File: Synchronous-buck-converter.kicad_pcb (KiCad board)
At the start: 2 copper layers, 107.2 x 56.3 mm, 84 parts, among them IC1 2EDF7275FXUMA2, IC2 LM5169PQDDARQ1, J1 Conn_01x02_Socket, J2 output, J4 RP2040 connector, Q1 IPP50R280CE, Q2 IPP50R280CE, U1 MGJ2D151505SC, U2 MGJ2D151505SC, U4 3.3V reg

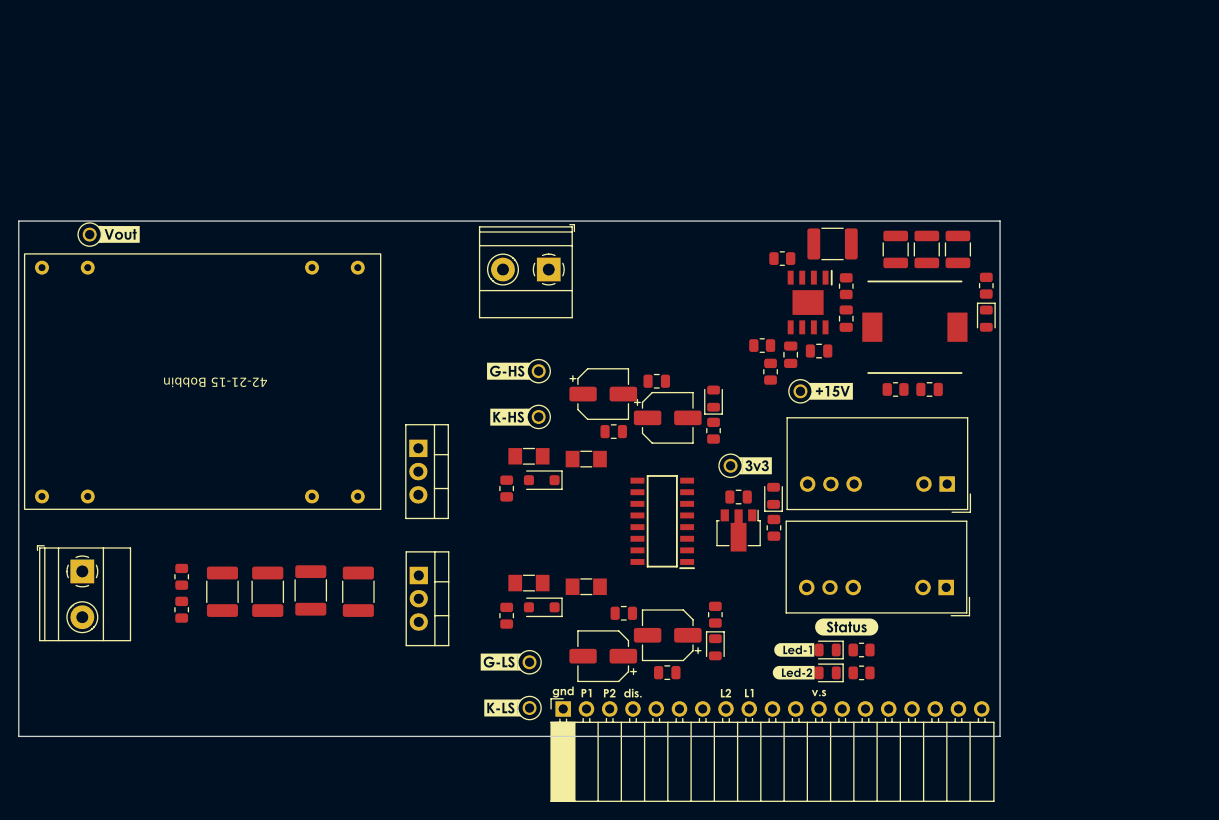
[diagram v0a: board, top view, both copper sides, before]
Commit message: V1
layout and tracing done
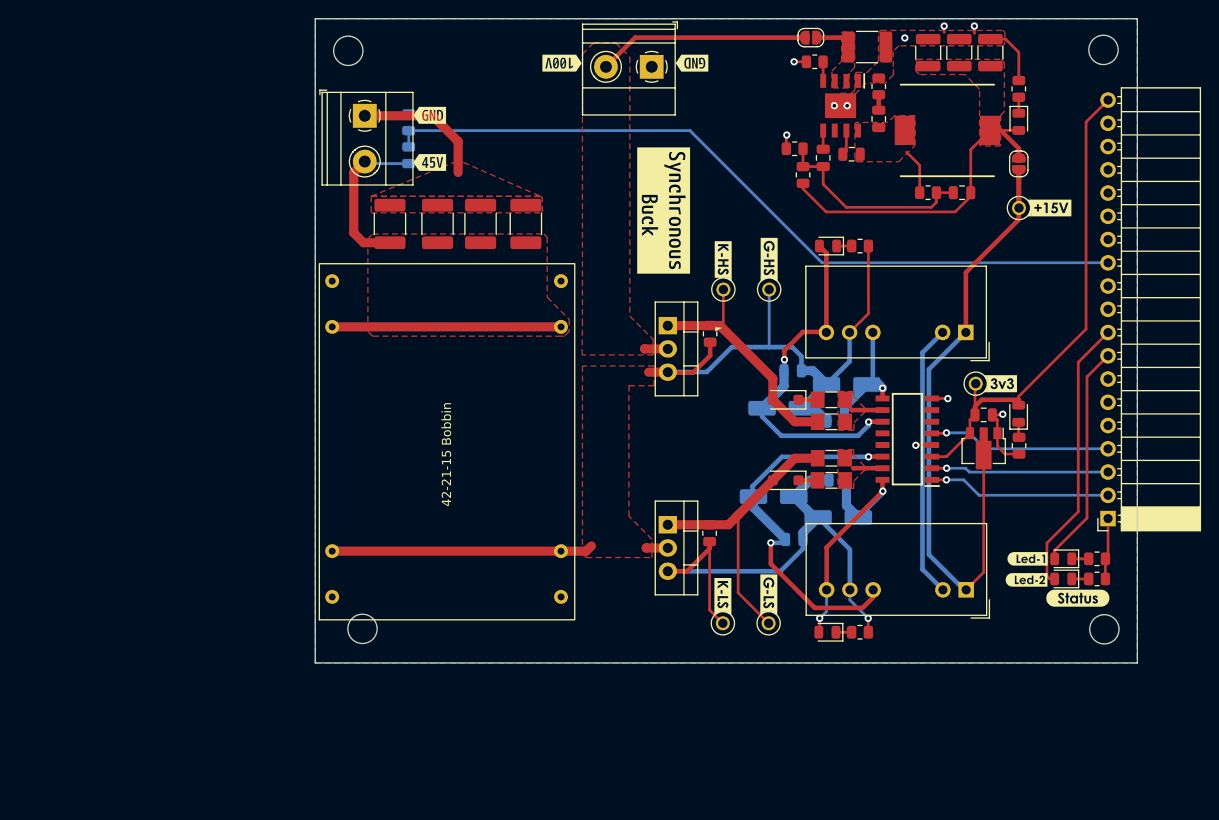
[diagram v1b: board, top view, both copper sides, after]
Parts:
- removed TP5: Vout, 5001 tp:KEYSTONE_5001
- removed kibuzzard-65CA698D: G***, kibuzzard-65CA698D
- removed kibuzzard-65CA6A14: G***, kibuzzard-65CA6A14
- removed kibuzzard-65CA6A3B: G***, kibuzzard-65CA6A3B
- removed kibuzzard-65CA6A4E: G***, kibuzzard-65CA6A4E
- removed kibuzzard-65CA6AA3: G***, kibuzzard-65CA6AA3
- removed kibuzzard-65CA6AAA: G***, kibuzzard-65CA6AAA
- removed kibuzzard-65CA6ABB: G***, kibuzzard-65CA6ABB
- removed kibuzzard-65CA6B07: G***, kibuzzard-65CA6B07
- added H1: MountingHole, MountingHole:MountingHole_3.2mm_M3, F.Cu at (120.0, 134.1)
- added H2: MountingHole, MountingHole:MountingHole_3.2mm_M3, F.Cu at (201.1, 134.1)
- added H3: MountingHole, MountingHole:MountingHole_3.2mm_M3, F.Cu at (118.5, 70.9)
- added H4: MountingHole, MountingHole:MountingHole_3.2mm_M3, F.Cu at (201.0, 70.8)
- added JP1: jumper, Jumper:SolderJumper-2_P1.3mm_Open_RoundedPad1.0x1.5mm, F.Cu at (169.0, 69.5)
- added JP2: jumper, Jumper:SolderJumper-2_P1.3mm_Open_RoundedPad1.0x1.5mm, F.Cu at (191.8, 83.2)
- added kibuzzard-65F43C21: G***, kibuzzard-65F43C21, F.Cu at (152.9, 88.3)
- added kibuzzard-65F43C4A: G***, kibuzzard-65F43C4A, F.Cu at (141.8, 72.2)
- added kibuzzard-65F43C74: G***, kibuzzard-65F43C74, F.Cu at (156.1, 72.2)
- added kibuzzard-65F43CE0: G***, kibuzzard-65F43CE0, F.Cu at (127.4, 83.1)
- added kibuzzard-65F43CF3: G***, kibuzzard-65F43CF3, F.Cu at (127.4, 78.0)
- added kibuzzard-65F44031: G***, kibuzzard-65F44031, F.Cu at (146.6, 88.3)
- added kibuzzard-65F4406D: G***, kibuzzard-65F4406D, F.Cu at (146.6, 116.5)
- C12, C13, C14, C15, C16, C17, C18, C19, R7, R8: moved to B.Cu
- moved J4 63.0 mm to (201.5, 122.0), turned to 180 degrees
- moved R8 58.7 mm to (125.1, 78.7), turned to 90 degrees
- moved J2 58.6 mm to (120.3, 78.0)
- moved R7 52.3 mm to (125.1, 82.3), turned to 90 degrees
- moved C4 52.1 mm to (137.9, 89.8), turned to 90 degrees
- moved C3 46.4 mm to (132.9, 89.8), turned to 90 degrees
- moved L1 45.2 mm to (143.2, 133.1), turned to 90 degrees
- moved C2 42.4 mm to (128.2, 89.8), turned to 90 degrees
- moved C1 40.3 mm to (123.0, 89.8), turned to 90 degrees
- moved R1 35.7 mm to (171.3, 115.4)
- moved R5 33.3 mm to (171.3, 111.4)
- moved kibuzzard-65CA6838 31.2 mm to (164.5, 93.5), turned to -90 degrees
- moved TP6 31.2 mm to (191.8, 88.1)
- moved kibuzzard-65CA6608 31.2 mm to (195.3, 88.1)
- moved kibuzzard-65CA6739 30.4 mm to (164.4, 130.1), turned to -90 degrees
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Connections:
- C1 pad 1: Net-(J2-Pin_1) -> Net-(J2-Pin_2)
- C2 pad 1: Net-(J2-Pin_1) -> Net-(J2-Pin_2)
- C3 pad 1: Net-(J2-Pin_1) -> Net-(J2-Pin_2)
- C4 pad 1: Net-(J2-Pin_1) -> Net-(J2-Pin_2)
- Cin1 pad 1: 100V -> Net-(IC2-EN/UVLO)
- IC2 pad 2: 100V -> Net-(IC2-EN/UVLO)
- IC2 pad 3: 100V -> Net-(IC2-EN/UVLO)
- J2 pad 1: Net-(J2-Pin_1) -> iso2-0V
- J2 pad 2: iso2-0V -> Net-(J2-Pin_2)
- J4 pad 2: PWM1 -> PWM2
- J4 pad 3: PWM2 -> PWM1
- L1 pad 2: Net-(J2-Pin_1) -> Net-(J2-Pin_2)
- Q1 pad 1: 100V -> Gate1
- Q1 pad 2: Gate1 -> 100V
- Q2 pad 1: iso1-0V -> Gate2
- Q2 pad 2: Gate2 -> iso1-0V
- R7 pad 1: Net-(J2-Pin_1) -> Net-(J2-Pin_2)
- TP6 pad 1: +15V -> Net-(JP2-B)
- U1 pad 1: +15V -> Net-(JP2-B)
- U2 pad 1: +15V -> Net-(JP2-B)
- U4 pad 2: +15V -> Net-(JP2-B)
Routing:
- net iso2-0V: track 0.00 -> 132.4 mm, vias 0 -> 11
- net iso1-0V: track 0.00 -> 91.4 mm
- net Vout-sense: track 0.00 -> 84.2 mm
- net Net-(JP2-B): track 0.00 -> 73.8 mm
- net +3.3V: track 0.00 -> 54.8 mm
- net Net-(J2-Pin_2): track 0.00 -> 42.6 mm
- net iso2-5V: track 0.00 -> 41.4 mm, vias 0 -> 2
- net iso1+15V: track 0.00 -> 38.3 mm, vias 0 -> 2
- net +15V: track 0.00 -> 36.9 mm
- net Gate2: track 0.00 -> 32.6 mm
- net Status-LED-2: track 0.00 -> 30.3 mm
- net iso2+15V: track 0.00 -> 28.2 mm, vias 0 -> 2
- net Gate1: track 0.00 -> 26.4 mm
- net 100V: track 0.00 -> 25.6 mm
- net Status-LED-1: track 0.00 -> 24.6 mm
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- added copper zone on F.Cu, net +15V
- added copper zone on F.Cu, net /auxiliary circuit/Vsw
- added copper zone on F.Cu, net 100V
- added copper zone on F.Cu, net Net-(IC1-OUTA)
- added copper zone on F.Cu, net Net-(IC1-OUTB)
- added copper zone on F.Cu, net Net-(IC2-EN/UVLO)
- added copper zone on F.Cu, net Net-(J2-Pin_2)
- added copper zone on F.Cu, net iso1-0V
- added copper zone on B.Cu, net iso2-0V
- added copper zone on F.Cu, net iso2-0V
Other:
- board size 107.2 x 56.3 mm -> 89.8 x 70.4 mm
